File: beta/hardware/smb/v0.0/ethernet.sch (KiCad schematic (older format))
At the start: 20 parts, among them J201 HR911105_RJ45, U201 ENC28J60, U301 74HC08, X201 25MHz

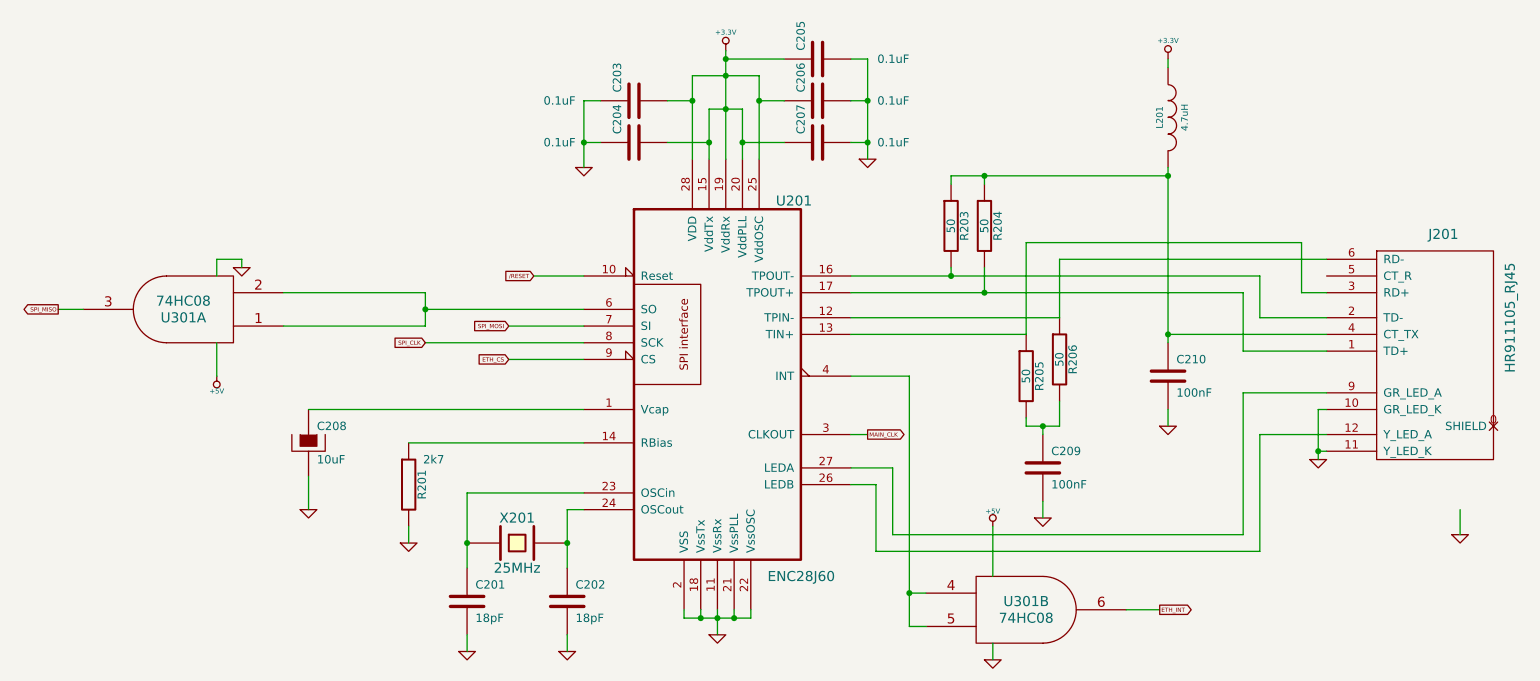
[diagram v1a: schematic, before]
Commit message: New components and corrections
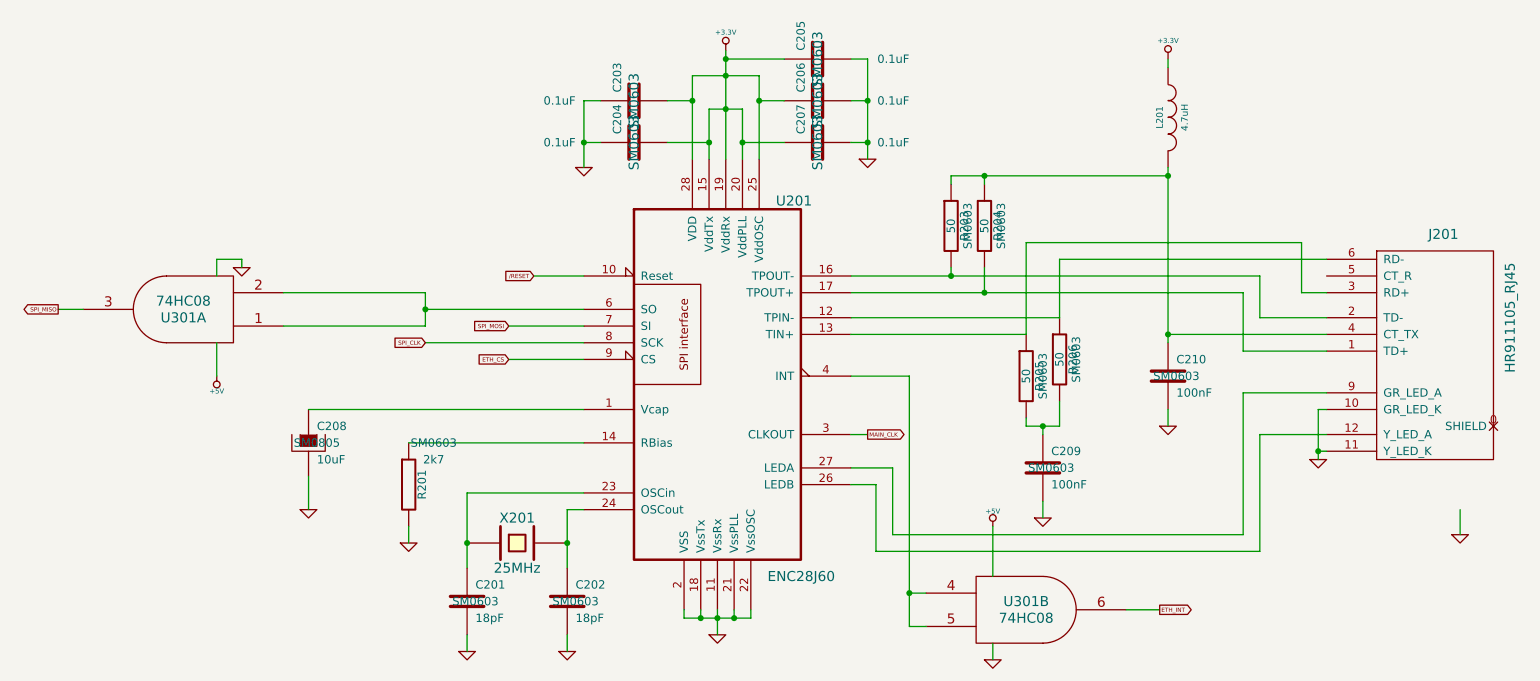
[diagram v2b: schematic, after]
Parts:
- C201, C202, C209, C210, R201, R203, R204, R205, R206: footprint (none) -> SM0603
- C208: footprint (none) -> SM0805
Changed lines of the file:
@@
-EESchema Schematic File Version 2  date 01/07/2012 23:30:37
+EESchema Schematic File Version 2  date 14/07/2012 20:45:27
 LIBS:power
 LIBS:device
@@
 LIBS:usd_conn
 LIBS:74lvc1g126gw
+LIBS:dual_self
 LIBS:SMB-cache
 EELAYER 25  0
@@
 Sheet 4 4
 Title ""
-Date "1 jul 2012"
+Date "14 jul 2012"
 Rev ""
 Comp ""
@@
 	7500 5000 7500 5100
 $Comp
-L +5V #PWR411
+L +5V #PWR060
 U 1 1 4FDE1BE4
 P 7500 4300
-F 0 "#PWR411" H 7500 4390 20  0001 C CNN
+F 0 "#PWR060" H 7500 4390 20  0001 C CNN
 F 1 "+5V" H 7500 4390 30  0000 C CNN
 	1    7500 4300
@@
 $EndComp
 $Comp
-L GND #PWR412
+L GND #PWR061
 U 1 1 4FDE1B8D
 P 7500 5100
-F 0 "#PWR412" H 7500 5100 30  0001 C CNN
+F 0 "#PWR061" H 7500 5100 30  0001 C CNN
 F 1 "GND" H 7500 5030 30  0001 C CNN
 	1    7500 5100
@@
 $EndComp
 $Comp
-L GND #PWR402
+L GND #PWR062
 U 1 1 4FDE1B70
 P 3000 2750
-F 0 "#PWR402" H 3000 2750 30  0001 C CNN
+F 0 "#PWR062" H 3000 2750 30  0001 C CNN
 F 1 "GND" H 3000 2680 30  0001 C CNN
 	1    3000 2750
@@
 $EndComp
 $Comp
-L +5V #PWR401
+L +5V #PWR063
 U 1 1 4FDE1B61
 P 2850 3400
-F 0 "#PWR401" H 2850 3490 20  0001 C CNN
+F 0 "#PWR063" H 2850 3490 20  0001 C CNN
 F 1 "+5V" H 2850 3490 30  0000 C CNN
 	1    2850 3400
@@
 F 0 "R204" V 7530 2500 50  0000 C CNN
 F 1 "50" V 7450 2500 50  0000 C CNN
+F 2 "SM0603" V 7550 2500 50  0000 C CNN
 	1    7450 2500
 	1    0    0    -1
@@
 F 0 "R203" V 7330 2500 50  0000 C CNN
 F 1 "50" V 7250 2500 50  0000 C CNN
+F 2 "SM0603" V 7350 2500 50  0000 C CNN
 	1    7250 2500
 	1    0    0    -1
@@
 $EndComp
 $Comp
-L +3.3V #PWR414
+L +3.3V #PWR064
 U 1 1 4FA00F89
 P 8550 1500
-F 0 "#PWR414" H 8550 1460 30  0001 C CNN
+F 0 "#PWR064" H 8550 1460 30  0001 C CNN
 F 1 "+3.3V" H 8550 1610 30  0000 C CNN
 	1    8550 1500
@@
 $EndComp
 $Comp
-L GND #PWR415
+L GND #PWR065
 U 1 1 4FA00F53
 P 8550 3700
-F 0 "#PWR415" H 8550 3700 30  0001 C CNN
+F 0 "#PWR065" H 8550 3700 30  0001 C CNN
 F 1 "GND" H 8550 3630 30  0001 C CNN
 	1    8550 3700
@@
 F 0 "C210" H 8600 3500 50  0000 L CNN
 F 1 "100nF" H 8600 3300 50  0000 L CNN
+F 2 "SM0603" H 8600 3400 50  0000 C CNN
 	1    8550 3400
 	1    0    0    -1
 $EndComp
 $Comp
-L GND #PWR416
+L GND #PWR066
 U 1 1 4FA00C7B
 P 9450 3900
-F 0 "#PWR416" H 9450 3900 30  0001 C CNN
+F 0 "#PWR066" H 9450 3900 30  0001 C CNN
 F 1 "GND" H 9450 3830 30  0001 C CNN
 	1    9450 3900
@@
 $EndComp
 $Comp
-L GND #PWR417
+L GND #PWR067
 U 1 1 4FA00C63
 P 10300 4350
-F 0 "#PWR417" H 10300 4350 30  0001 C CNN
+F 0 "#PWR067" H 10300 4350 30  0001 C CNN
 F 1 "GND" H 10300 4280 30  0001 C CNN
 	1    10300 4350
@@
 $EndComp
 $Comp
-L GND #PWR413
+L GND #PWR068
 U 1 1 4F9FF676
 P 7800 4250
-F 0 "#PWR413" H 7800 4250 30  0001 C CNN
+F 0 "#PWR068" H 7800 4250 30  0001 C CNN
 F 1 "GND" H 7800 4180 30  0001 C CNN
 	1    7800 4250
@@
 F 0 "C209" H 7850 4050 50  0000 L CNN
 F 1 "100nF" H 7850 3850 50  0000 L CNN
+F 2 "SM0603" H 7850 3950 50  0000 C CNN
 	1    7800 3950
 	1    0    0    -1
@@
 F 0 "R206" V 7980 3300 50  0000 C CNN
 F 1 "50" V 7900 3300 50  0000 C CNN
+F 2 "SM0603" V 8000 3300 50  0000 C CNN
 	1    7900 3300
 	1    0    0    -1
@@
 F 0 "R205" V 7780 3400 50  0000 C CNN
 F 1 "50" V 7700 3400 50  0000 C CNN
+F 2 "SM0603" V 7800 3400 50  0000 C CNN
 	1    7700 3400
 	1    0    0    -1
@@
 SPI_CLK
 $Comp
-L GND #PWR403
+L GND #PWR069
 U 1 1 4F9FEE21
 P 3400 4200
-F 0 "#PWR403" H 3400 4200 30  0001 C CNN
+F 0 "#PWR069" H 3400 4200 30  0001 C CNN
 F 1 "GND" H 3400 4130 30  0001 C CNN
 	1    3400 4200
@@
 $EndComp
 $Comp
-L GND #PWR404
+L GND #PWR070
 U 1 1 4F9FEE1E
 P 4000 4400
-F 0 "#PWR404" H 4000 4400 30  0001 C CNN
+F 0 "#PWR070" H 4000 4400 30  0001 C CNN
 F 1 "GND" H 4000 4330 30  0001 C CNN
 	1    4000 4400
@@
 F 0 "R201" V 4080 4050 50  0000 C CNN
 F 1 "2k7" H 4150 4200 50  0000 C CNN
+F 2 "SM0603" H 4150 4300 50  0000 C CNN
 	1    4000 4050
 	1    0    0    -1
@@
 F 0 "C208" H 3450 3900 50  0000 L CNN
 F 1 "10uF" H 3450 3700 50  0000 L CNN
+F 2 "SM0805" H 3450 3800 50  0000 C CNN
 	1    3400 3800
 	1    0    0    -1
 $EndComp
 $Comp
-L GND #PWR407
+L GND #PWR071
 U 1 1 4F9FC462
 P 5050 2150
-F 0 "#PWR407" H 5050 2150 30  0001 C CNN
+F 0 "#PWR071" H 5050 2150 30  0001 C CNN
 F 1 "GND" H 5050 2080 30  0001 C CNN
 	1    5050 2150
@@
 $EndComp
 $Comp
-L GND #PWR410
+L GND #PWR072
 U 1 1 4F9FC45C
 P 6750 2100
-F 0 "#PWR410" H 6750 2100 30  0001 C CNN
+F 0 "#PWR072" H 6750 2100 30  0001 C CNN
 F 1 "GND" H 6750 2030 30  0001 C CNN
 	1    6750 2100
@@
 F 0 "C203" H 5400 1850 50  0000 L CNN
 F 1 "0.1uF" V 5350 2100 50  0000 L CNN
-F 2 "SM0603" H 5350 1750 60  0001 C CNN
+F 2 "SM0603" H 5350 1750 60  0000 C CNN
 	1    5350 1750
 	0    -1   -1   0
@@
 F 0 "C204" H 5400 2100 50  0000 L CNN
 F 1 "0.1uF" V 5350 2350 50  0000 L CNN
-F 2 "SM0603" H 5350 2000 60  0001 C CNN
+F 2 "SM0603" H 5350 2000 60  0000 C CNN
 	1    5350 2000
 	0    -1   -1   0
@@
 F 0 "C207" H 6500 2100 50  0000 L CNN
 F 1 "0.1uF" V 6450 1450 50  0000 L CNN
-F 2 "SM0603" H 6450 2000 60  0001 C CNN
+F 2 "SM0603" H 6450 2000 60  0000 C CNN
 	1    6450 2000
 	0    -1   -1   0
@@
 F 0 "C206" H 6500 1850 50  0000 L CNN
 F 1 "0.1uF" V 6450 1200 50  0000 L CNN
-F 2 "SM0603" H 6450 1750 60  0001 C CNN
+F 2 "SM0603" H 6450 1750 60  0000 C CNN
 	1    6450 1750
 	0    -1   -1   0
@@
 F 0 "C205" H 6500 1600 50  0000 L CNN
 F 1 "0.1uF" V 6450 950 50  0000 L CNN
-F 2 "SM0603" H 6450 1500 60  0001 C CNN
+F 2 "SM0603" H 6450 1500 60  0000 C CNN
 	1    6450 1500
 	0    -1   -1   0
 $EndComp
 $Comp
-L +3.3V #PWR409
+L +3.3V #PWR073
 U 1 1 4F9FC2EE
 P 5900 1450
-F 0 "#PWR409" H 5900 1410 30  0001 C CNN
+F 0 "#PWR073" H 5900 1410 30  0001 C CNN
 F 1 "+3.3V" H 5900 1560 30  0000 C CNN
 	1    5900 1450
@@
 $EndComp
 $Comp
-L GND #PWR405
+L GND #PWR074
 U 1 1 4F9D7261
 P 4350 5050
-F 0 "#PWR405" H 4350 5050 30  0001 C CNN
+F 0 "#PWR074" H 4350 5050 30  0001 C CNN
 F 1 "GND" H 4350 4980 30  0001 C CNN
 	1    4350 5050
@@
 $EndComp
 $Comp
-L GND #PWR406
+L GND #PWR075
 U 1 1 4F9D725B
 P 4950 5050
-F 0 "#PWR406" H 4950 5050 30  0001 C CNN
+F 0 "#PWR075" H 4950 5050 30  0001 C CNN
 F 1 "GND" H 4950 4980 30  0001 C CNN
 	1    4950 5050
@@
 F 0 "C202" H 5000 4850 50  0000 L CNN
 F 1 "18pF" H 5000 4650 50  0000 L CNN
+F 2 "SM0603" H 5000 4750 50  0000 C CNN
 	1    4950 4750
 	1    0    0    -1
@@
 F 0 "C201" H 4400 4850 50  0000 L CNN
 F 1 "18pF" H 4400 4650 50  0000 L CNN
+F 2 "SM0603" H 4400 4750 50  0000 C CNN
 	1    4350 4750
 	1    0    0    -1
@@
 $EndComp
 $Comp
-L GND #PWR408
+L GND #PWR076
 U 1 1 4F9D6E29
 P 5850 4950
-F 0 "#PWR408" H 5850 4950 30  0001 C CNN
+F 0 "#PWR076" H 5850 4950 30  0001 C CNN
 F 1 "GND" H 5850 4880 30  0001 C CNN
 	1    5850 4950

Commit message: All footprint ready
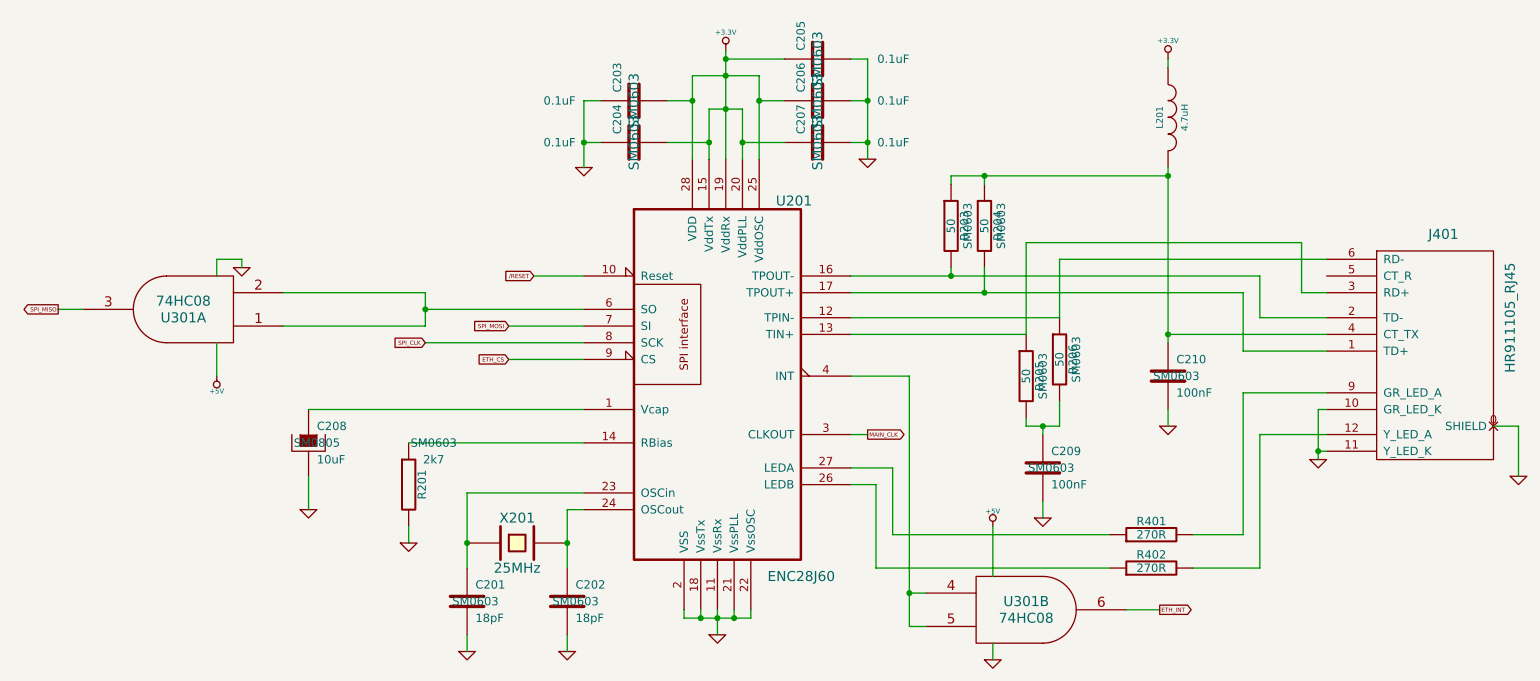
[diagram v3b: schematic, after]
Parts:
- removed J201: HR911105_RJ45, symbol HR911105_RJ45
- added J401: HR911105_RJ45, symbol HR911105_RJ45
- added R401, R402: 270R, symbol R
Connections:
- net GND: now also J401.0 (SHIELD), J401.10 (GR_LED_K), J401.11 (Y_LED_K)
- net at R206.1, U201.12 (TPIN-): now also J401.6 (RD-)
- net at R205.1, U201.13 (TIN+): now also J401.3 (RD+)
- net at R203.2, U201.16 (TPOUT-): now also J401.2 (TD-)
- net at R204.2, U201.17 (TPOUT+): now also J401.1 (TD+)
- net at U201.26 (LEDB): now also R402.1
- net at U201.27 (LEDA): now also R401.1
- net at C210.1, L201.2, R203.1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: now also J401.4 (CT_TX)
- new net: J401.9 (GR_LED_A), R401.2
- new net: J401.12 (Y_LED_A), R402.2
